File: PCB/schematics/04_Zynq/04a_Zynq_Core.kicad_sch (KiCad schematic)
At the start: 133 parts, among them U26 xczu4evfbvb900pkg

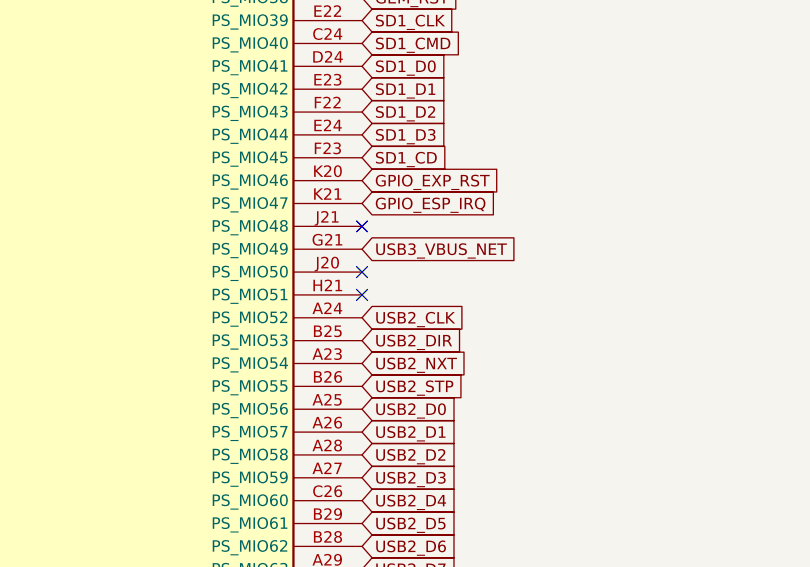
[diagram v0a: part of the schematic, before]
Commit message: feat: Section 4 Done
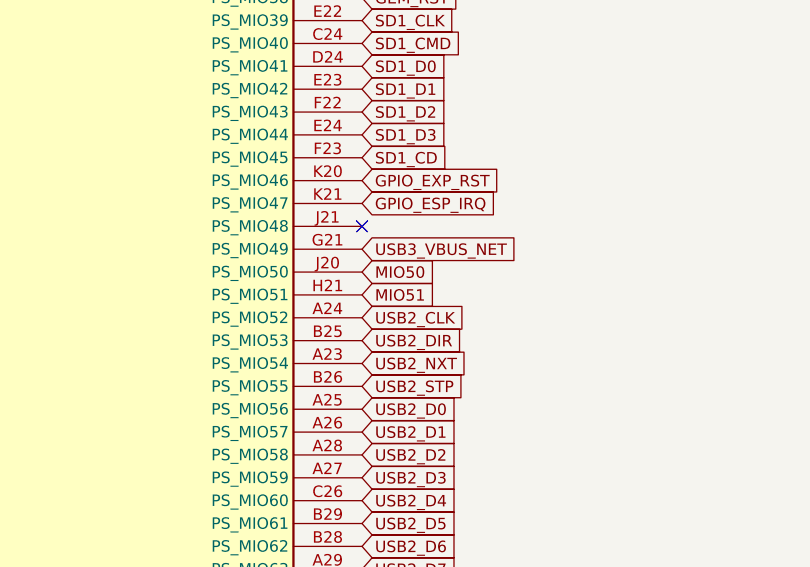
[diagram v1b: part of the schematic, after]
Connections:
- net MIO51: now reaches U26.H21 (PS_MIO51)
- net MIO50: now reaches U26.J20 (PS_MIO50)
- no-connect marks 278 -> 276
